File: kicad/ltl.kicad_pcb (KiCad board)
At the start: 2 copper layers, 77.7 x 48 mm, 20 parts, among them J1 CONN_01X03, U1 TP4056, U2 ESP-12E, U3 DS18B20

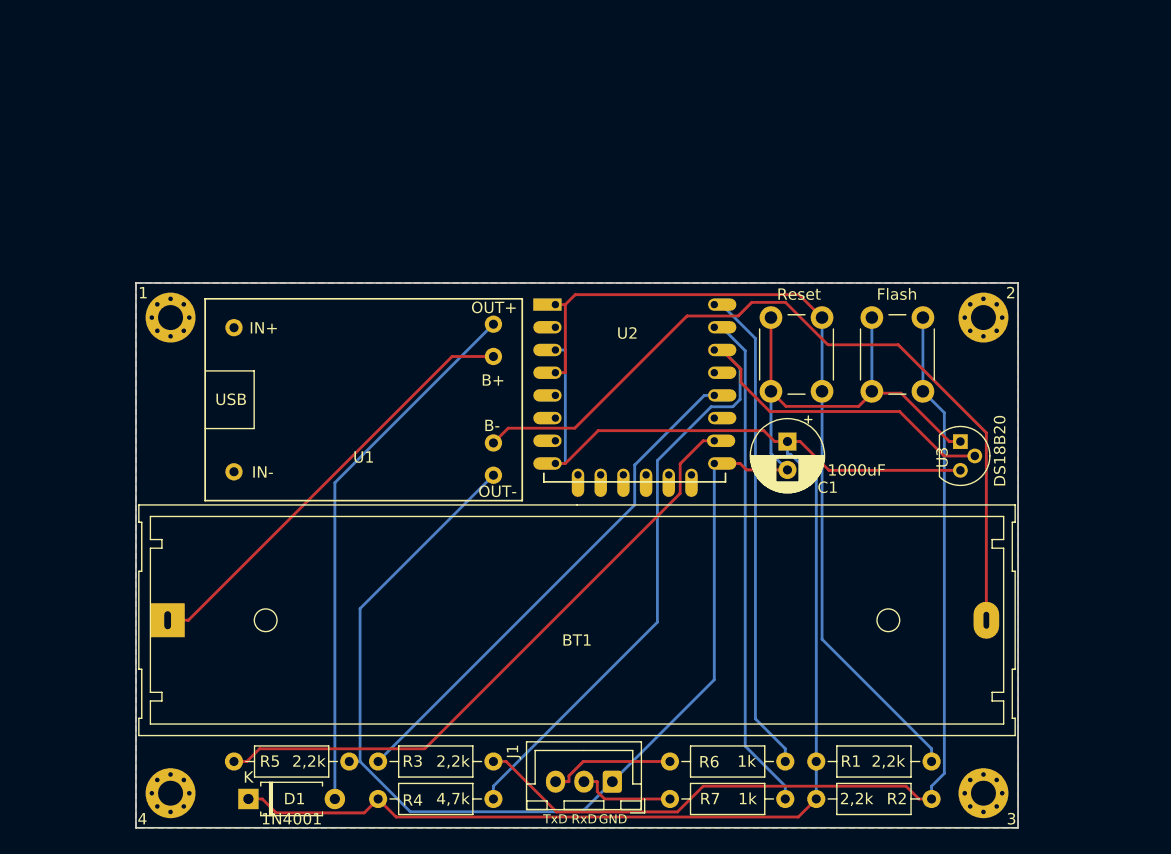
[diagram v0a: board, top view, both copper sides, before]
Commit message: Lots of added features and bug fixes
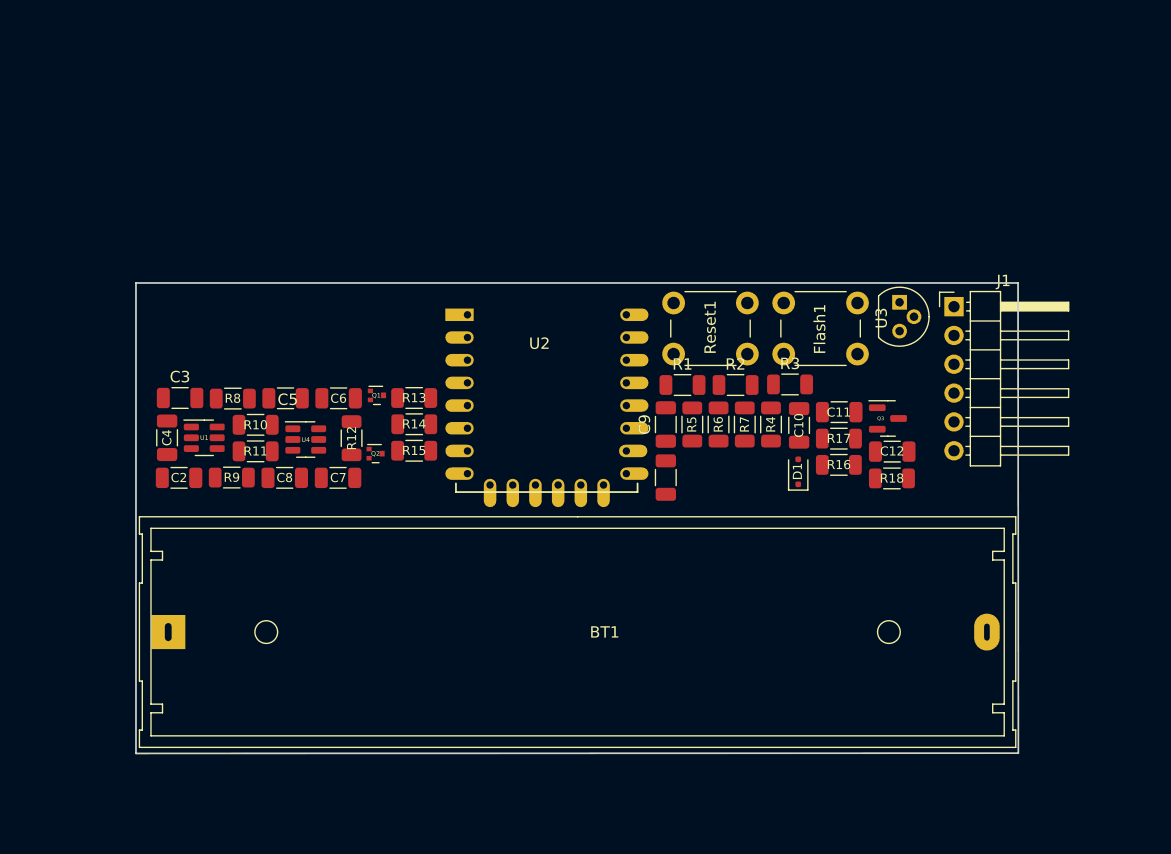
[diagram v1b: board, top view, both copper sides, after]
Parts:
- removed MH_1: 1, MountingHole:MountingHole_2.2mm_M2_Pad_Via
- removed MH_2: 2, MountingHole:MountingHole_2.2mm_M2_Pad_Via
- removed MH_3: 3, MountingHole:MountingHole_2.2mm_M2_Pad_Via
- removed MH_4: 4, MountingHole:MountingHole_2.2mm_M2_Pad_Via
- added C10: 10uF, Capacitor_SMD:C_1206_3216Metric, F.Cu at (144.5, 103.5)
- added C11: 10uF, Capacitor_SMD:C_1206_3216Metric, F.Cu at (148.1, 102.3)
- added C12: 10uF, Capacitor_SMD:C_1206_3216Metric, F.Cu at (152.7, 105.8)
- added C2: 10uF, Capacitor_SMD:C_1206_3216Metric, F.Cu at (89.9, 108.1)
- added C3: 10uF, Capacitor_SMD:C_1206_3216Metric, F.Cu at (90.0, 101.1)
- added C4: 100nF, Capacitor_SMD:C_1206_3216Metric, F.Cu at (88.8, 104.6)
- added C5: 10uF, Capacitor_SMD:C_1206_3216Metric, F.Cu at (99.3, 101.1)
- added C6: 100nF, Capacitor_SMD:C_1206_3216Metric, F.Cu at (104.0, 101.1)
- added C7: 10uF, Capacitor_SMD:C_1206_3216Metric, F.Cu at (103.9, 108.1)
- added C8: 100nF, Capacitor_SMD:C_1206_3216Metric, F.Cu at (99.2, 108.1)
- added C9: 100nF, Capacitor_SMD:C_1206_3216Metric, F.Cu at (132.8, 103.4)
- added Q1: RUM001L02T2CL, Package_TO_SOT_SMD:SOT-723, F.Cu at (107.3, 100.8)
- added Q2: RZM001P02T2L, Package_TO_SOT_SMD:SOT-723, F.Cu at (107.2, 106.0)
- added Q3: BC857, Package_TO_SOT_SMD:SOT-23, F.Cu at (152.4, 102.9)
- added R10: 10k, Resistor_SMD:R_1206_3216Metric, F.Cu at (96.6, 103.4)
- added R11: 10k, Resistor_SMD:R_1206_3216Metric, F.Cu at (96.6, 105.8)
- added R12: 10k, Resistor_SMD:R_1206_3216Metric, F.Cu at (105.1, 104.6)
- added R13: 10k, Resistor_SMD:R_1206_3216Metric, F.Cu at (110.6, 101.1)
- added R14: 49.9k, Resistor_SMD:R_1206_3216Metric, F.Cu at (110.6, 103.4)
- added R15: 10k, Resistor_SMD:R_1206_3216Metric, F.Cu at (110.6, 105.7)
- added R16: 100, Resistor_SMD:R_1206_3216Metric, F.Cu at (148.0, 107.0)
- added R17: 100, Resistor_SMD:R_1206_3216Metric, F.Cu at (148.0, 104.6)
- added R18: 10k, Resistor_SMD:R_1206_3216Metric, F.Cu at (152.7, 108.2)
- added R8: 42k, Resistor_SMD:R_1206_3216Metric, F.Cu at (94.6, 101.1)
- added R9: 10k, Resistor_SMD:R_1206_3216Metric, F.Cu at (94.5, 108.1)
- added U4: TPS73733DCQR, Package_TO_SOT_SMD:SOT-23-6, F.Cu at (101.1, 104.7)
- C1: value 1000uF -> 10uF; footprint Capacitor_THT:CP_Radial_D6.3mm_P2.50mm -> Capacitor_SMD:C_1206_3216Metric
- D1: value 1N4001 -> BAT54J; footprint Diode_THT:D_A-405_P7.62mm_Horizontal -> Diode_SMD:D_SOD-323F
- J1: value CONN_01X03 -> Conn_01x06; footprint Connector_JST:JST_XH_B3B-XH-A_1x03_P2.50mm_Vertical -> Connector_PinHeader_2.54mm:PinHeader_1x06_P2.54mm_Horizontal
- R1, R2, R3, R5: value 2,2k -> 10k; footprint Resistor_THT:R_Axial_DIN0207_L6.3mm_D2.5mm_P10.16mm_Horizontal -> Resistor_SMD:R_1206_3216Metric
- R4, R6, R7: footprint Resistor_THT:R_Axial_DIN0207_L6.3mm_D2.5mm_P10.16mm_Horizontal -> Resistor_SMD:R_1206_3216Metric
- U1: value TP4056 -> TPL5111; footprint TP4506:TP4056 -> Package_TO_SOT_SMD:SOT-23-6
- moved D1 56.4 mm to (144.5, 107.6), turned to 90 degrees
- moved J1 51.6 mm to (158.2, 93.0), turned to 0 degrees
- moved R3 49.2 mm to (143.7, 99.9)
- moved R4 47.8 mm to (142.1, 103.4), turned to 90 degrees
- moved R5 42.4 mm to (135.1, 103.4), turned to 90 degrees
- moved R2 37.2 mm to (138.9, 99.9)
- moved R1 35.2 mm to (134.3, 99.9)
- moved R7 33.6 mm to (139.8, 103.4), turned to 90 degrees
- moved R6 30.0 mm to (137.4, 103.4), turned to -90 degrees
- moved U1 14.4 mm to (92.1, 104.6)
- moved U3 13.4 mm to (153.4, 92.6)
- moved Flash1 12.3 mm to (143.2, 92.7), turned to 0 degrees
- moved C1 11.2 mm to (132.8, 108.1)
- moved U2 7.80 mm to (115.3, 93.7)
- moved Reset1 7.32 mm to (140.0, 97.2), turned to 180 degrees
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- renumbered Flash to Flash1, Reset to Reset1
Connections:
- net Net-(R3-Pad1) renamed GPIO0
- BT1 pad 1: Net-(BT1-Pad1) -> +4V
- BT1 pad 2: Net-(BT1-Pad2) -> GND
- D1 pad 1: +3V3 -> DTR
- D1 pad 2: Net-(D1-Pad2) -> Net-(D1-A)
- J1 pad 1: GND -> DTR
- J1 pad 2: /RxD -> /TxD
- J1 pad 3: /TxD -> /RxD
- R1 pad 2: Net-(R1-Pad2) -> RESET
- R4 pad 2: Net-(R4-Pad2) -> Net-(U2-GPIO4)
- R5 pad 1: GND -> +3V3
- R5 pad 2: Net-(R5-Pad2) -> Net-(U2-CH_PD)
- Reset1 pad 1: Net-(R1-Pad2) -> RESET
- U1 pad 1: Net-(U1-Pad1) -> +4V
- U1 pad 2: Net-(U1-Pad2) -> GND
- U1 pad 3: Net-(D1-Pad2) -> Net-(U1-DELAY/M_DRV)
- U1 pad 4: Net-(BT1-Pad1) -> Net-(U1-DONE)
- U1 pad 5: Net-(BT1-Pad2) -> Net-(U1-~{DRV})
- U1 pad 6: GND -> +4V
- U2 pad 1: Net-(R1-Pad2) -> RESET
- U2 pad 10: Net-(R5-Pad2) -> DONE
- U2 pad 11: Net-(U2-Pad11) -> unconnected-(U2-GPIO2-Pad11)
- U2 pad 13: Net-(U2-Pad13) -> Net-(U2-GPIO4)
- U2 pad 14: Net-(R4-Pad2) -> unconnected-(U2-GPIO5-Pad14)
- U2 pad 17: Net-(U2-Pad17) -> unconnected-(U2-CS0-Pad17)
- U2 pad 18: Net-(U2-Pad18) -> unconnected-(U2-MISO-Pad18)
- U2 pad 19: Net-(U2-Pad19) -> unconnected-(U2-GPIO9-Pad19)
- U2 pad 2: Net-(U2-Pad2) -> BAT_DIV
- U2 pad 20: Net-(U2-Pad20) -> unconnected-(U2-GPIO10-Pad20)
- U2 pad 21: Net-(U2-Pad21) -> unconnected-(U2-MOSI-Pad21)
- U2 pad 22: Net-(U2-Pad22) -> unconnected-(U2-SCLK-Pad22)
- U2 pad 3: +3V3 -> Net-(U2-CH_PD)
- U2 pad 4: Net-(R1-Pad2) -> unconnected-(U2-GPIO16-Pad4)
- U2 pad 5: Net-(U2-Pad5) -> unconnected-(U2-GPIO14-Pad5)
- U2 pad 6: Net-(U2-Pad6) -> unconnected-(U2-GPIO12-Pad6)
- U2 pad 7: Net-(U2-Pad7) -> unconnected-(U2-GPIO13-Pad7)
- U3 pad 2: Net-(R4-Pad2) -> Net-(U2-GPIO5)
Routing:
- net +3V3: track 135.2 -> 0.00 mm
- net GND: track 134.8 -> 0.00 mm
- net Net-(Flash1-Pad1): track 85.5 -> 0.00 mm
- net Net-(R4-Pad2): track 78.5 -> 0.00 mm
- net Net-(R1-Pad2): track 74.7 -> 0.00 mm
- net Net-(BT1-Pad2): track 69.8 -> 0.00 mm
- net Net-(R5-Pad2): track 55.6 -> 0.00 mm
- net Net-(D1-Pad2): track 47.6 -> 0.00 mm
- net GPIO0: track 45.0 -> 0.00 mm
- net Net-(U2-RXD): track 44.5 -> 0.00 mm
- net Net-(U2-TXD): track 43.2 -> 0.00 mm
- net Net-(BT1-Pad1): track 38.3 -> 0.00 mm
- net /TxD: track 11.1 -> 0.00 mm
- net /RxD: track 8.73 -> 0.00 mm
- removed copper zone on B.Cu, net (none)
- removed copper zone on F.Cu, net GND
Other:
- board size 77.7 x 48 mm -> 77.7 x 41.5 mm
- board text added: "Rev.2.0 Lfd.Nr."
- board text removed: "GND"
- board text removed: "Rev.1.2 Lfd.Nr."
- board text removed: "RxD"
- board text removed: "TxD"

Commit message: Latest PCB version, sent for production
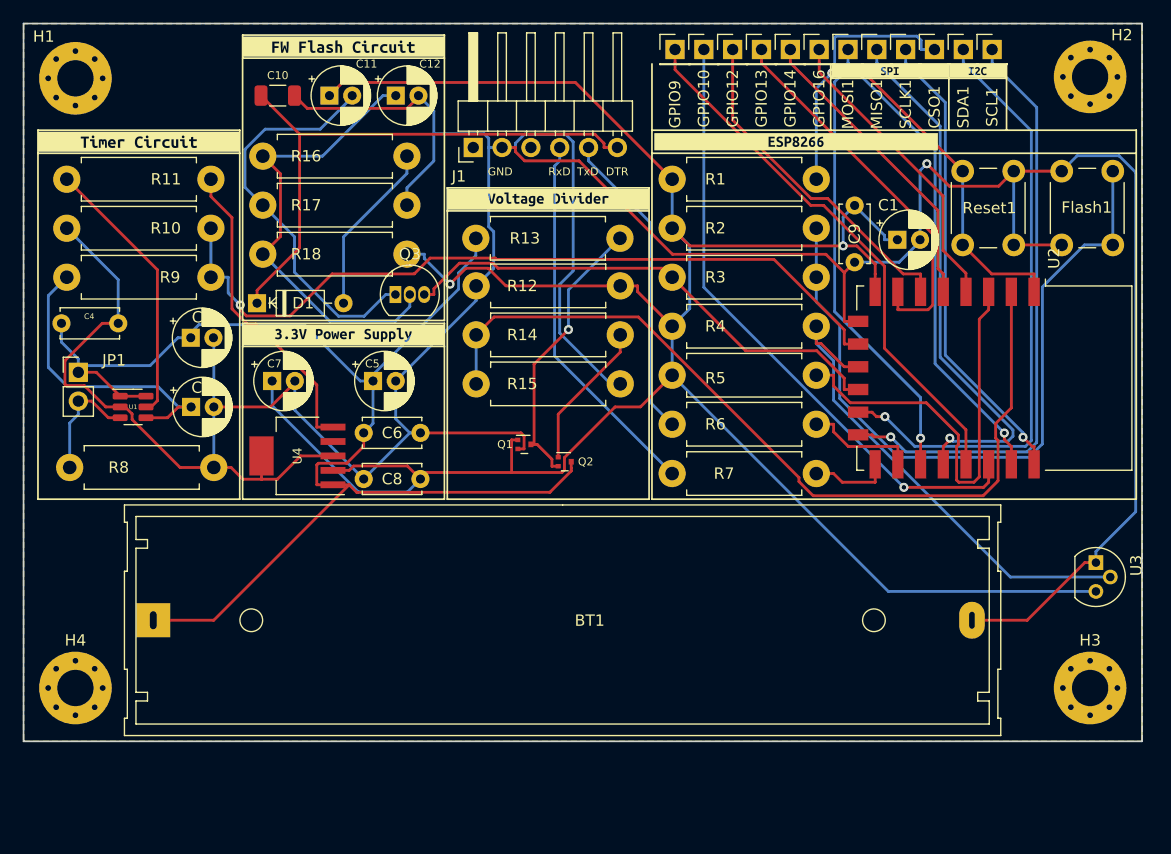
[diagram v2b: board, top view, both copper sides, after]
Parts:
- added CSO1: CSO, Connector_PinHeader_2.54mm:PinHeader_1x01_P2.54mm_Vertical, F.Cu at (156.5, 70.4)
- added GPIO10: GPIO10, Connector_PinHeader_2.54mm:PinHeader_1x01_P2.54mm_Vertical, F.Cu at (136.1, 70.4)
- added GPIO12: GPIO12, Connector_PinHeader_2.54mm:PinHeader_1x01_P2.54mm_Vertical, F.Cu at (138.7, 70.4)
- added GPIO13: GPIO13, Connector_PinHeader_2.54mm:PinHeader_1x01_P2.54mm_Vertical, F.Cu at (141.2, 70.4)
- added GPIO14: GPIO14, Connector_PinHeader_2.54mm:PinHeader_1x01_P2.54mm_Vertical, F.Cu at (143.8, 70.4)
- added GPIO16: GPIO16, Connector_PinHeader_2.54mm:PinHeader_1x01_P2.54mm_Vertical, F.Cu at (146.3, 70.4)
- added GPIO9: GPIO9, Connector_PinHeader_2.54mm:PinHeader_1x01_P2.54mm_Vertical, F.Cu at (133.6, 70.4)
- added H1: MountingHole, MountingHole:MountingHole_3.2mm_M3_Pad_Via, F.Cu at (80.8, 72.9)
- added H2: MountingHole, MountingHole:MountingHole_3.2mm_M3_Pad_Via, F.Cu at (170.2, 72.8)
- added H3: MountingHole, MountingHole:MountingHole_3.2mm_M3_Pad_Via, F.Cu at (170.2, 126.6)
- added H4: MountingHole, MountingHole:MountingHole_3.2mm_M3_Pad_Via, F.Cu at (80.8, 126.6)
- added JP1: JP1, Connector_PinHeader_2.54mm:PinHeader_1x02_P2.54mm_Vertical, F.Cu at (81.0, 98.8)
- added MISO1: MISO, Connector_PinHeader_2.54mm:PinHeader_1x01_P2.54mm_Vertical, F.Cu at (151.4, 70.4)
- added MOSI1: MOSI, Connector_PinHeader_2.54mm:PinHeader_1x01_P2.54mm_Vertical, F.Cu at (148.8, 70.4)
- added SCL1: SCL, Connector_PinHeader_2.54mm:PinHeader_1x01_P2.54mm_Vertical, F.Cu at (161.5, 70.4)
- added SCLK1: SCLK, Connector_PinHeader_2.54mm:PinHeader_1x01_P2.54mm_Vertical, F.Cu at (153.9, 70.4)
- added SDA1: SDA, Connector_PinHeader_2.54mm:PinHeader_1x01_P2.54mm_Vertical, F.Cu at (159.0, 70.4)
- added kibuzzard-65989638: G***, kibuzzard-65989638, F.Cu at (152.5, 72.3)
- added kibuzzard-65989978: G***, kibuzzard-65989978, F.Cu at (86.4, 78.5)
- added kibuzzard-65989B2E: G***, kibuzzard-65989B2E, F.Cu at (104.4, 95.5)
- added kibuzzard-65989B49: G***, kibuzzard-65989B49, F.Cu at (122.4, 83.6)
- added kibuzzard-65989BDF: G***, kibuzzard-65989BDF, F.Cu at (160.3, 72.3)
- added kibuzzard-65991234: G***, kibuzzard-65991234, F.Cu at (144.3, 78.5)
- added kibuzzard-659AB4FF: G***, kibuzzard-659AB4FF, F.Cu at (104.4, 70.1)
- C1, C11, C12, C2, C3, C5, C7: footprint Capacitor_SMD:C_1206_3216Metric -> Capacitor_THT:CP_Radial_D5.0mm_P2.00mm
- C4, C6, C8, C9: footprint Capacitor_SMD:C_1206_3216Metric -> Capacitor_THT:C_Disc_D5.0mm_W2.5mm_P5.00mm
- D1: value BAT54J -> BAT85; footprint Diode_SMD:D_SOD-323F -> Diode_THT:D_DO-35_SOD27_P7.62mm_Horizontal
- J1: value Conn_01x06 -> J1
- Q3: value BC857 -> BC327; footprint Package_TO_SOT_SMD:SOT-23 -> Package_TO_SOT_THT:TO-92_Inline
- R1, R10, R11, R12, R13, R14, R15, R16, R17, R18, R2, R3, R4, R5, R6, R7, R8, R9: footprint Resistor_SMD:R_1206_3216Metric -> Resistor_THT:R_Axial_DIN0411_L9.9mm_D3.6mm_P12.70mm_Horizontal
- U2: footprint ESP8266:ESP-12E -> RF_Module:ESP-12E
- U4: footprint Package_TO_SOT_SMD:SOT-23-6 -> Package_TO_SOT_SMD:SOT-223-6
- moved R18 58.9 mm to (97.3, 88.4)
- moved R16 57.6 mm to (97.3, 79.8), turned to 0 degrees
- moved R17 54.8 mm to (97.3, 84.1)
- moved C10 54.4 mm to (98.6, 74.4), turned to 0 degrees
- moved C12 53.8 mm to (109.0, 74.4)
- moved C11 52.9 mm to (103.2, 74.4)
- moved D1 49.9 mm to (96.8, 92.7), turned to 0 degrees
- moved U2 46.8 mm to (161.7, 99.3), turned to -90 degrees
- moved Q3 44.7 mm to (109.0, 91.9)
- moved J1 44.6 mm to (115.8, 79.0), turned to 90 degrees
- moved Flash1 31.2 mm to (172.2, 81.1), turned to -90 degrees
- moved C1 29.2 mm to (153.2, 87.1), turned to 0 degrees
- moved R11 29.2 mm to (80.0, 81.8)
- moved U3 28.7 mm to (170.7, 115.6)
- moved C9 25.5 mm to (149.4, 84.1), turned to -90 degrees
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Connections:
- net Net-(U1-DELAY/M_DRV) renamed DELAY
- C10 pad 2: RESET -> GND
- C11 pad 1: Net-(Q3-C) -> +3V3
- C11 pad 2: +3V3 -> Net-(Q3-C)
- C12 pad 1: GND -> Net-(Q3-B)
- C12 pad 2: Net-(Q3-B) -> GND
- J1 pad 1: DTR -> unconnected-(J1-Pin_1-Pad1)
- J1 pad 2: /TxD -> GND
- J1 pad 3: /RxD -> unconnected-(J1-Pin_3-Pad3)
- J1 pad 4: unconnected-(J1-Pin_4-Pad4) -> /RxD
- J1 pad 5: GND -> /TxD
- J1 pad 6: unconnected-(J1-Pin_6-Pad6) -> DTR
- Q3 pad 1: Net-(Q3-B) -> Net-(Q3-C)
- Q3 pad 2: GPIO0 -> Net-(Q3-B)
- Q3 pad 3: Net-(Q3-C) -> FLASH
- R16 pad 1: Net-(D1-A) -> Net-(Q3-B)
- R16 pad 2: Net-(Q3-B) -> Net-(D1-A)
- R17 pad 1: GND -> Net-(Q3-C)
- R17 pad 2: Net-(Q3-C) -> GND
- R3 pad 1: GPIO0 -> FLASH
- R4 pad 2: Net-(U2-GPIO4) -> Net-(U2-GPIO2)
- U2 pad 11: unconnected-(U2-GPIO2-Pad11) -> Net-(U2-GPIO2)
- U2 pad 12: GPIO0 -> FLASH
- U2 pad 13: Net-(U2-GPIO4) -> Net-(SDA1-Pin_1)
- U2 pad 14: unconnected-(U2-GPIO5-Pad14) -> Net-(SCL1-Pin_1)
- U2 pad 17: unconnected-(U2-CS0-Pad17) -> Net-(CSO1-Pin_1)
- U2 pad 18: unconnected-(U2-MISO-Pad18) -> Net-(MISO1-Pin_1)
- U2 pad 19: unconnected-(U2-GPIO9-Pad19) -> Net-(GPIO9-Pin_1)
- U2 pad 20: unconnected-(U2-GPIO10-Pad20) -> Net-(GPIO10-Pin_1)
- U2 pad 21: unconnected-(U2-MOSI-Pad21) -> Net-(MOSI1-Pin_1)
- U2 pad 22: unconnected-(U2-SCLK-Pad22) -> Net-(SCLK1-Pin_1)
- U2 pad 4: unconnected-(U2-GPIO16-Pad4) -> Net-(GPIO16-Pin_1)
- U2 pad 5: unconnected-(U2-GPIO14-Pad5) -> Net-(GPIO14-Pin_1)
- U2 pad 6: unconnected-(U2-GPIO12-Pad6) -> Net-(GPIO12-Pin_1)
- U2 pad 7: unconnected-(U2-GPIO13-Pad7) -> Net-(GPIO13-Pin_1)
- U3 pad 2: Net-(U2-GPIO5) -> Net-(U2-GPIO2)
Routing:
- net GND: track 0.00 -> 324.2 mm, vias 0 -> 1
- net +3V3: track 0.00 -> 213.8 mm, vias 0 -> 2
- net +4V: track 0.00 -> 117.4 mm
- net BAT_DIV: track 0.00 -> 75.5 mm
- net DONE: track 0.00 -> 70.1 mm, vias 0 -> 1
- net Net-(Flash1-Pad1): track 0.00 -> 64.4 mm
- net Net-(GPIO10-Pin_1): track 0.00 -> 55.1 mm, vias 0 -> 1
- net Net-(SDA1-Pin_1): track 0.00 -> 53.7 mm, vias 0 -> 1
- net Net-(SCL1-Pin_1): track 0.00 -> 52.9 mm, vias 0 -> 1
- net Net-(CSO1-Pin_1): track 0.00 -> 50.9 mm, vias 0 -> 1
- net DTR: track 0.00 -> 50.0 mm
- net Net-(GPIO9-Pin_1): track 0.00 -> 47.8 mm
- net Net-(MISO1-Pin_1): track 0.00 -> 47.5 mm, vias 0 -> 1
- net FLASH: track 0.00 -> 44.9 mm
- net Net-(U2-GPIO2): track 0.00 -> 44.1 mm
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- added copper zone on B.Cu, net GND
- added copper zone on F.Cu, net GND
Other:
- board size 77.7 x 41.5 mm -> 98.6 x 63.2 mm
- board text added: "DTR"
- board text added: "GND"
- board text added: "RxD"
- board text added: "TxD"
